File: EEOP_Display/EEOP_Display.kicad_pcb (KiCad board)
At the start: 2 copper layers, 18 x 26.7 mm, 4 parts, among them J1 FH34SRJ-32S-0.5SH_50_, J2 Conn_01x32

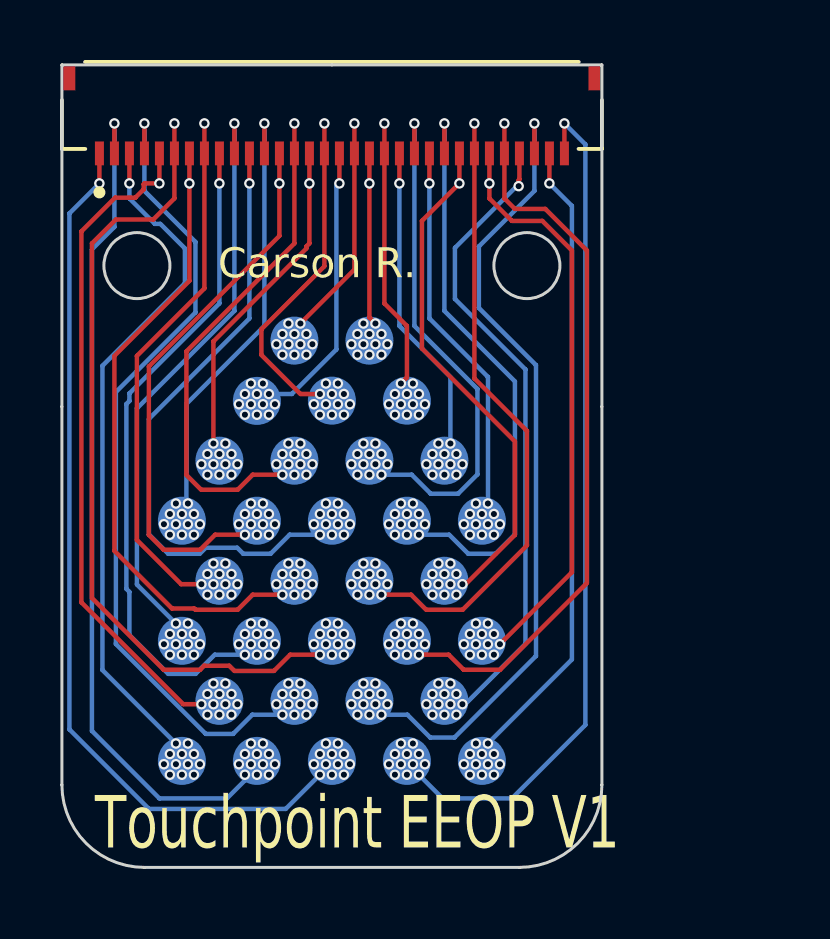
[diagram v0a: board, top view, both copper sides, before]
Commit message: Final manufacturing adjustments
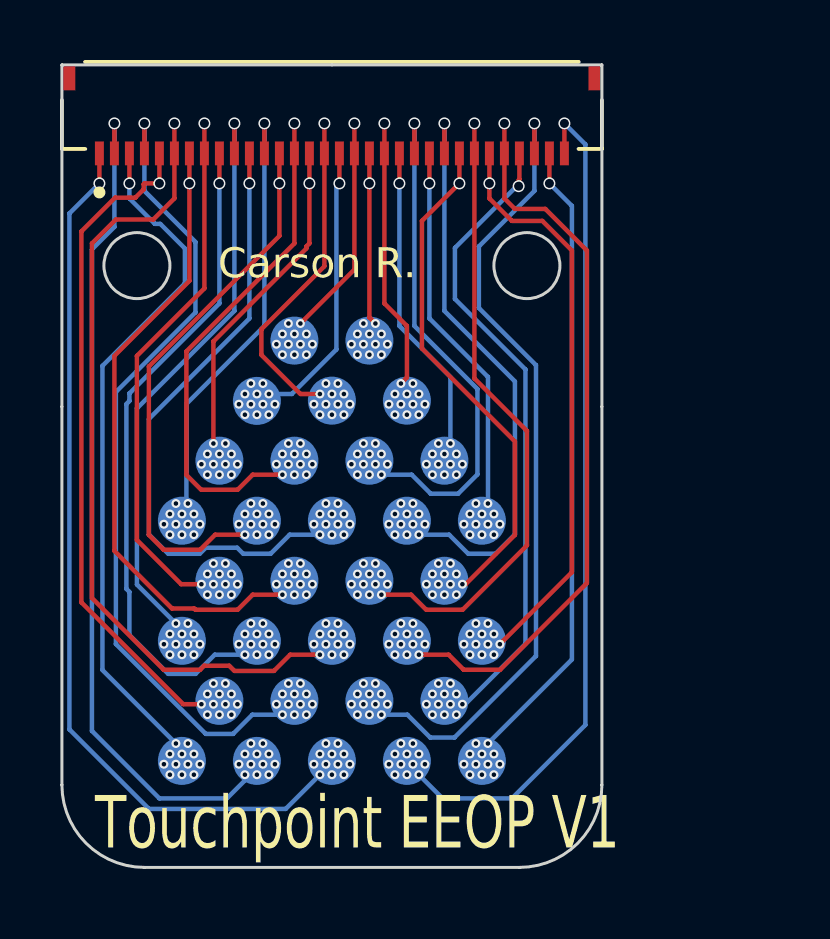
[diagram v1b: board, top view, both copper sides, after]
